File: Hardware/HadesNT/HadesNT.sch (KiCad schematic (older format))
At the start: 98 parts, among them J1 USB_B_Micro, J10 Conn_02x08_Odd_Even, J11 Conn_01x08, J2 Conn_01x02, J3 Conn_02x05_Odd_Even, J4 Conn_01x04, J5 Conn_01x04, J6 Conn_01x04, J7 Conn_01x04, J8 Conn_01x06, J9 Conn_01x02, Q1 AO4407A, Q2 MMBT3904, Q3 MMBT3904, Q4 MMBT3904, Q5 MMBT3904, Q6 MMBT3904, Q7 MMBT3904, U1 INA219AIDCNR, U2 MP2451DT-LF-Z, U3 SRV05-4, U4 W25Q128JVS, U5 BMP280, U6 BMX055, U7 STM32H750VBT6, Y1 16 MHz

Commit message: EKF STM32F4 testbed.
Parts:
- added D8: RE, LED_SMD:LED_0603_1608Metric, symbol Device:LED_Small
- added R25: 2k2, Resistor_SMD:R_0603_1608Metric, symbol Device:R_Small
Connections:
- net ACC_INT: now also U7.90 (PB4); no longer U7.8 (PC14-OSC32_IN)
- net GND: now also R25.1
- net GYR_INT: now also U7.91 (PB5); no longer U7.7 (PC13)
- net LED_A: now also U7.81 (PD0); no longer U7.90 (PB4)
- net LED_B: now also U7.82 (PD1); no longer U7.91 (PB5)
- net MAG_INT: now also U6.10 (INT5), U7.35 (PB1); no longer U6.2 (DRDYM), U7.9 (PC15-OSC32_OUT)
- net MAGD_DRDY: now reaches U7.34 (PB0)
- net MAGD_DRDY: now also U6.2 (DRDYM)
- net at R24.2, S1.B1 (COM): now also D8.2 (A)
- net TIM3_CH1 renamed TIM8_CH1
- net TIM3_CH2 renamed TIM8_CH2
- net TIM3_CH3 renamed TIM8_CH3
- net TIM3_CH4 renamed TIM8_CH4
- new net: D8.1 (K), R25.2
- no-connect marks 43 -> 41
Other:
- moved on the sheet: C12, C13, R24

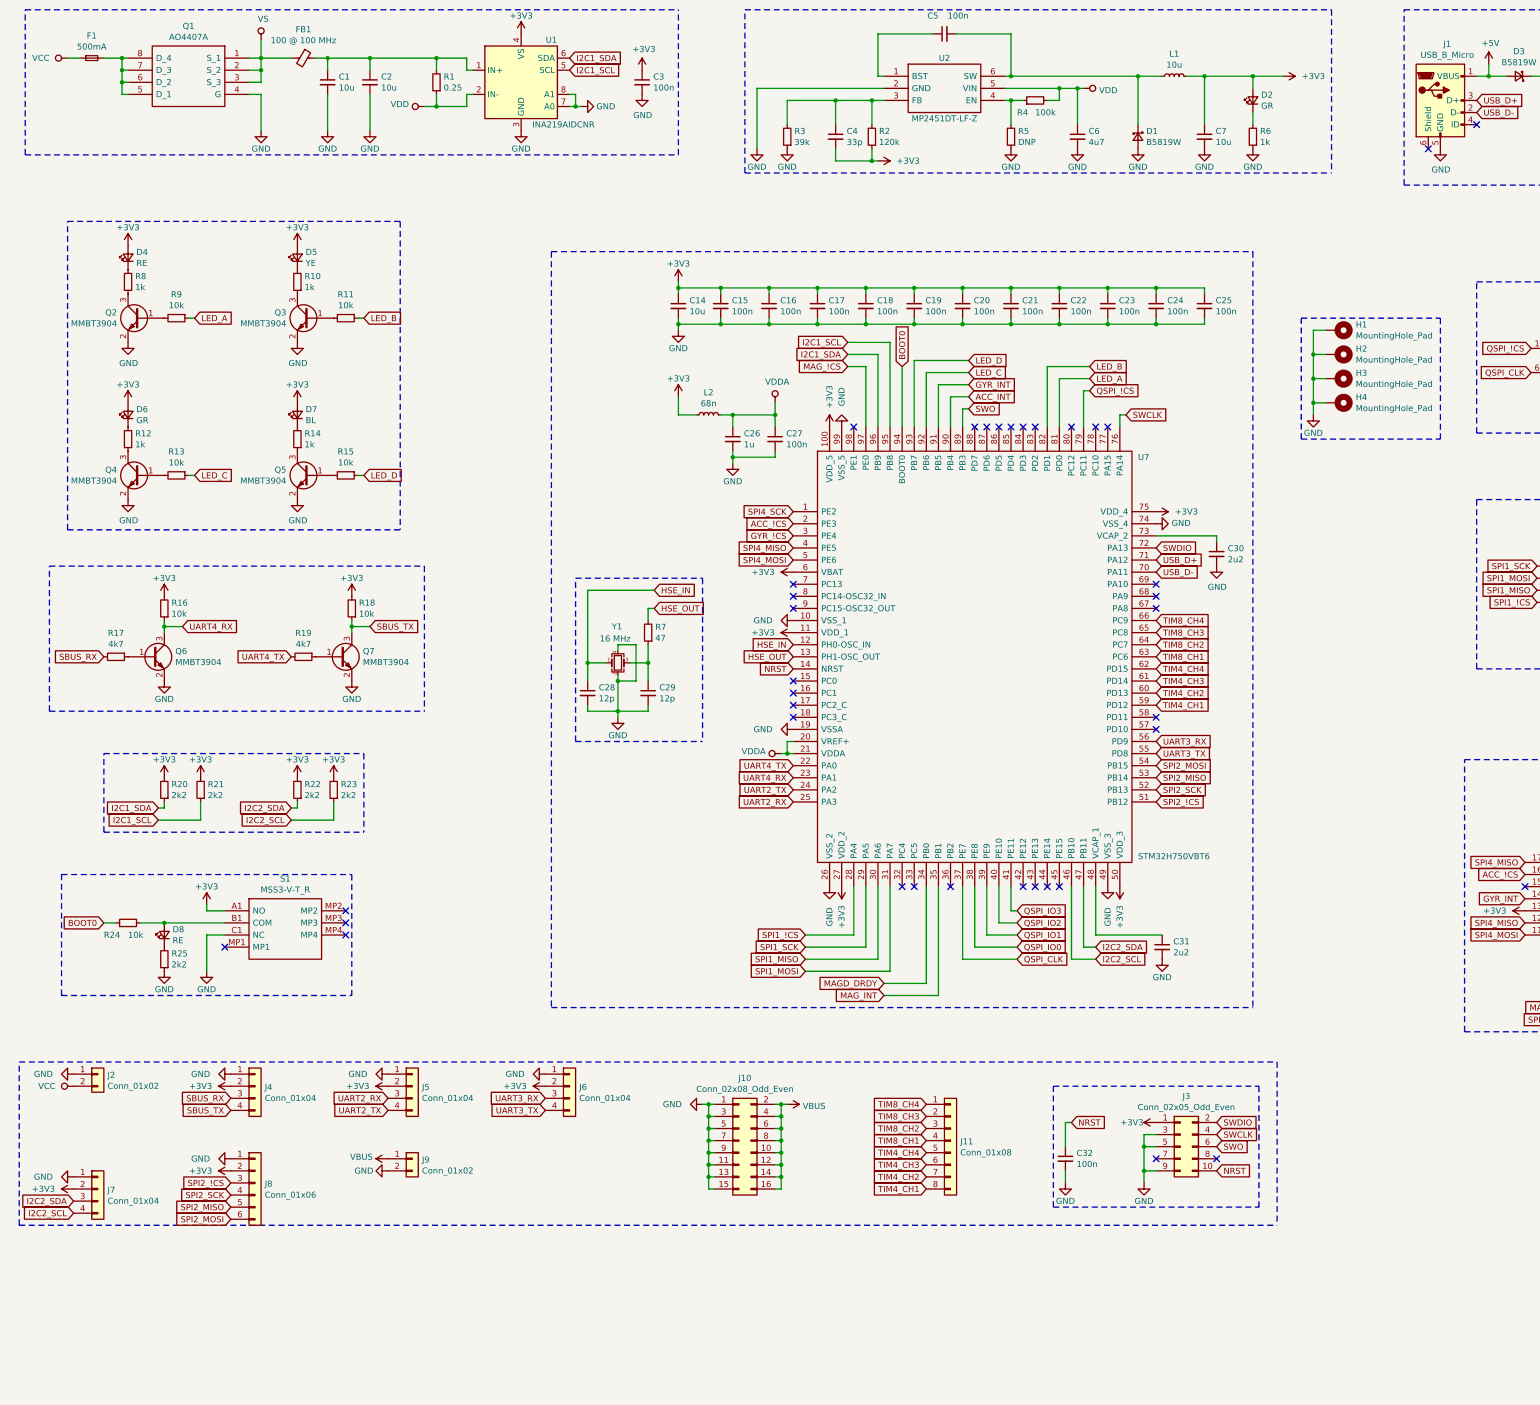
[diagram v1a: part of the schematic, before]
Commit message: Finished HadesNT.
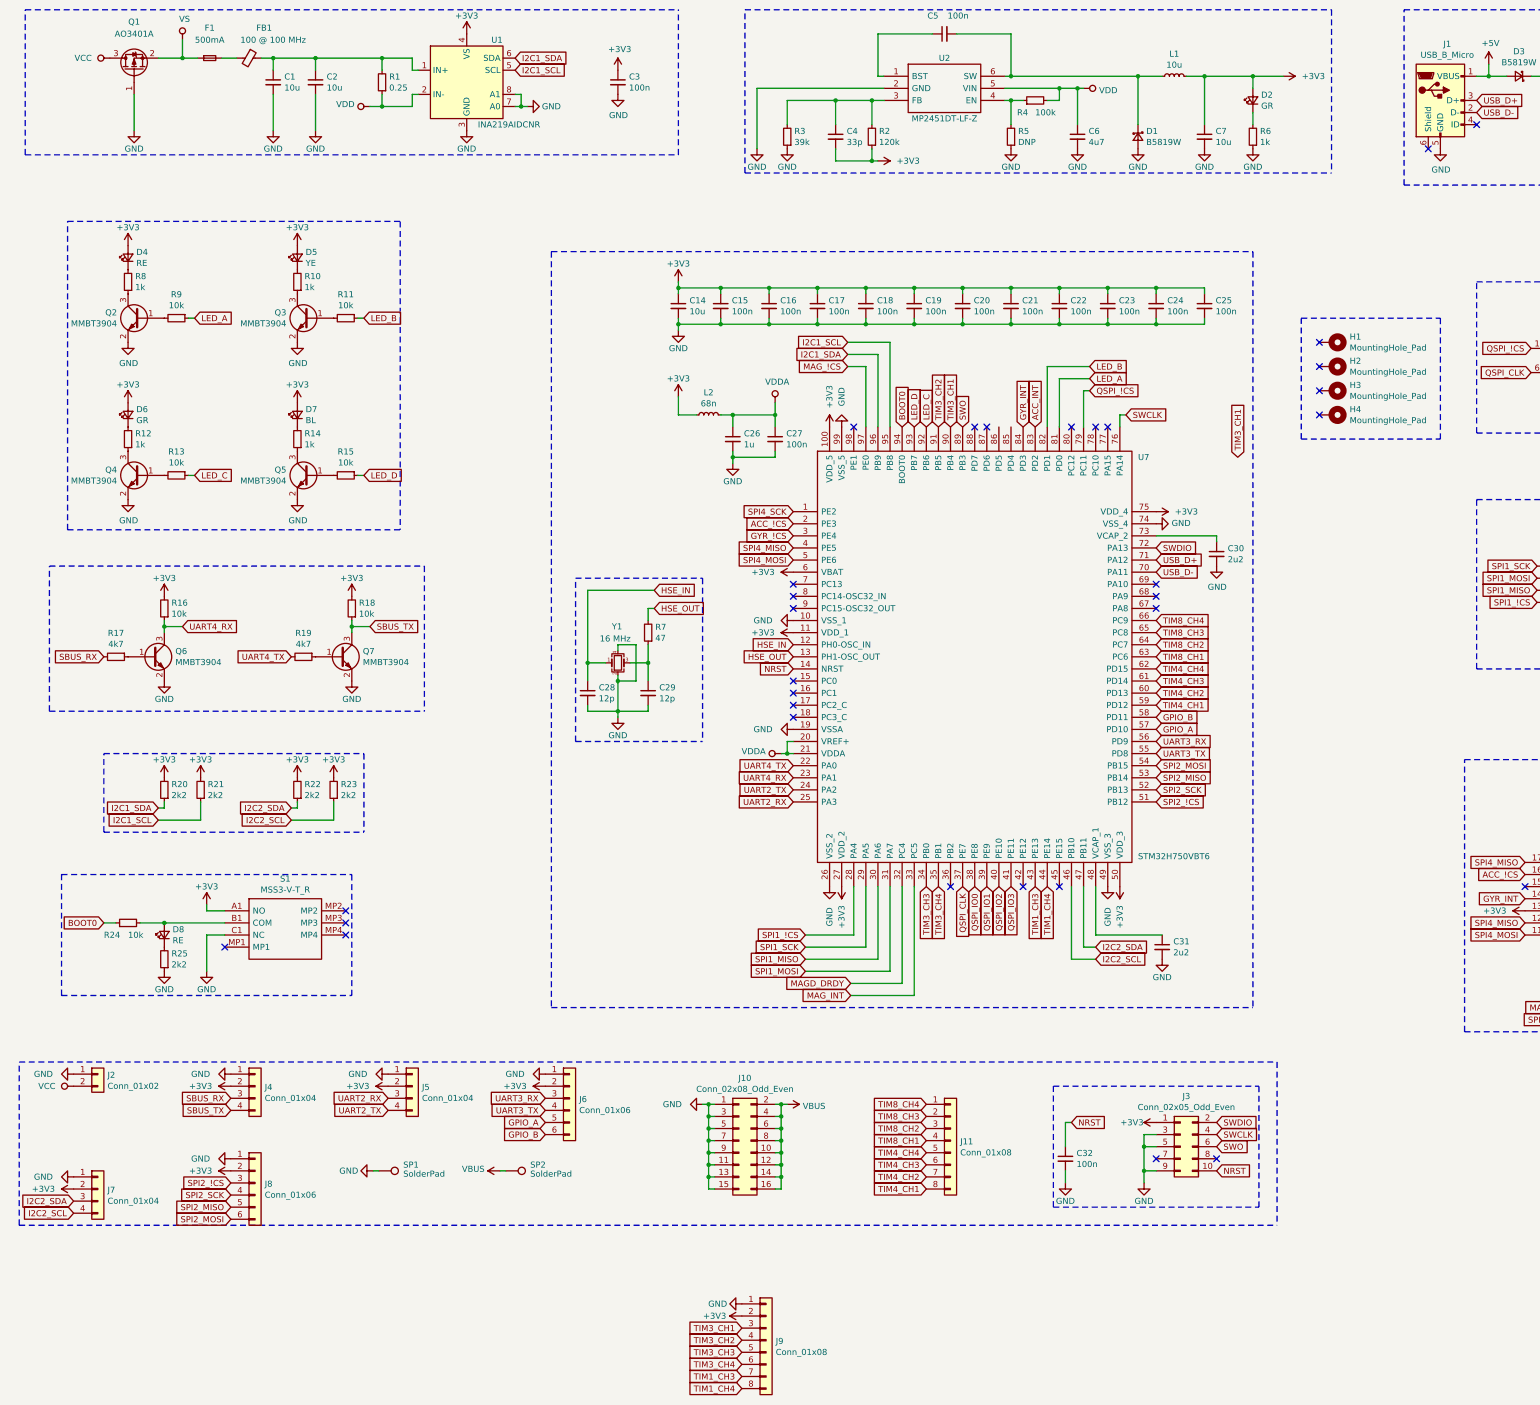
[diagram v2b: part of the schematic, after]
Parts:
- removed J6: Conn_01x04, Connector_JST:JST_GH_SM04B-GHS-TB_1x04-1MP_P1.25mm_Horizontal, symbol Connector_Generic:Conn_01x04
- removed J9: Conn_01x02, TerminalBlock_Phoenix:TerminalBlock_Phoenix_PT-1,5-2-3.5-H_1x02_P3.50mm_Horizontal, symbol Connector_Generic:Conn_01x02
- removed Q1: AO4407A, AO4407A:SOIC127P600X175-8N, symbol AO4407A:AO4407A
- added J6: Conn_01x06, Connector_JST:JST_GH_SM06B-GHS-TB_1x06-1MP_P1.25mm_Horizontal, symbol Connector_Generic:Conn_01x06
- added J9: Conn_01x08, Connector_JST:JST_GH_SM08B-GHS-TB_1x08-1MP_P1.25mm_Horizontal, symbol Connector_Generic:Conn_01x08
- added Q1: AO3401A, Package_TO_SOT_SMD:SOT-23, symbol Transistor_FET:AO3401A
- added SP1, SP2: SolderPad, TestPoint:TestPoint_Pad_2.0x2.0mm, symbol Connector:TestPoint
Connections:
- net +3V3: now also J6.2 (Pin_2), J9.2 (Pin_2)
- net ACC_INT: now also U7.83 (PD2); no longer U7.90 (PB4)
- net GND: now also J6.1 (Pin_1), J9.1 (Pin_1), Q1.1 (G), SP1.1; no longer H1.1, H2.1, H3.1, H4.1
- net GYR_INT: now also U7.84 (PD3); no longer U7.91 (PB5)
- net MAGD_DRDY: now also U7.32 (PC4); no longer U7.34 (PB0)
- net MAG_INT: now also U7.33 (PC5); no longer U7.35 (PB1)
- net UART3_RX: now also J6.3 (Pin_3)
- net UART3_TX: now also J6.4 (Pin_4)
- net VBUS: now also SP2.1
- net VCC: now also Q1.3 (D); no longer F1.1
- net VS: now also F1.1, Q1.2 (S); no longer FB1.2
- net TIM1_CH3: now reaches U7.43 (PE13)
- net TIM1_CH3: now also J9.7 (Pin_7)
- net TIM1_CH4: now reaches U7.44 (PE14)
- net TIM1_CH4: now also J9.8 (Pin_8)
- net GPIO_A: now reaches U7.57 (PD10)
- net GPIO_A: now also J6.5 (Pin_5)
- net GPIO_B: now reaches U7.58 (PD11)
- net GPIO_B: now also J6.6 (Pin_6)
- net at F1.2: now also FB1.2
- new net TIM3_CH1: J9.3 (Pin_3), U7.90 (PB4)
- new net TIM3_CH2: J9.4 (Pin_4), U7.91 (PB5)
- new net TIM3_CH3: J9.5 (Pin_5), U7.34 (PB0)
- new net TIM3_CH4: J9.6 (Pin_6), U7.35 (PB1)
- no-connect marks 41 -> 35
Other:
- moved on the sheet: C1, C2, C3, F1, FB1, H1, H2, H3, H4, R1, U1
